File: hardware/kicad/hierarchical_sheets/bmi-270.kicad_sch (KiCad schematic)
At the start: 3 parts

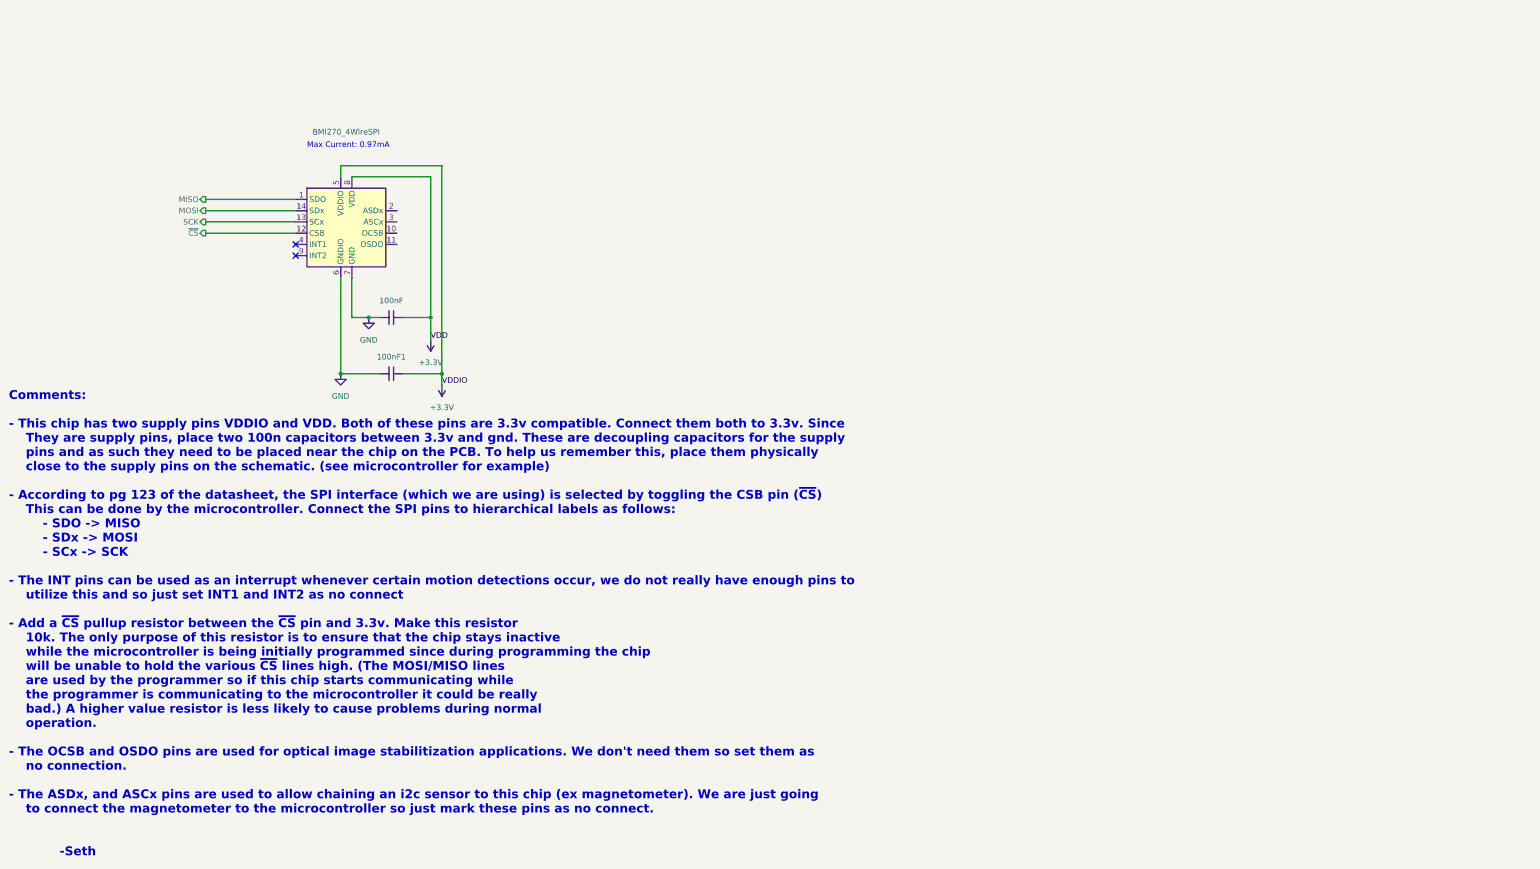
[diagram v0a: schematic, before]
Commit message: Finnished Schematic?
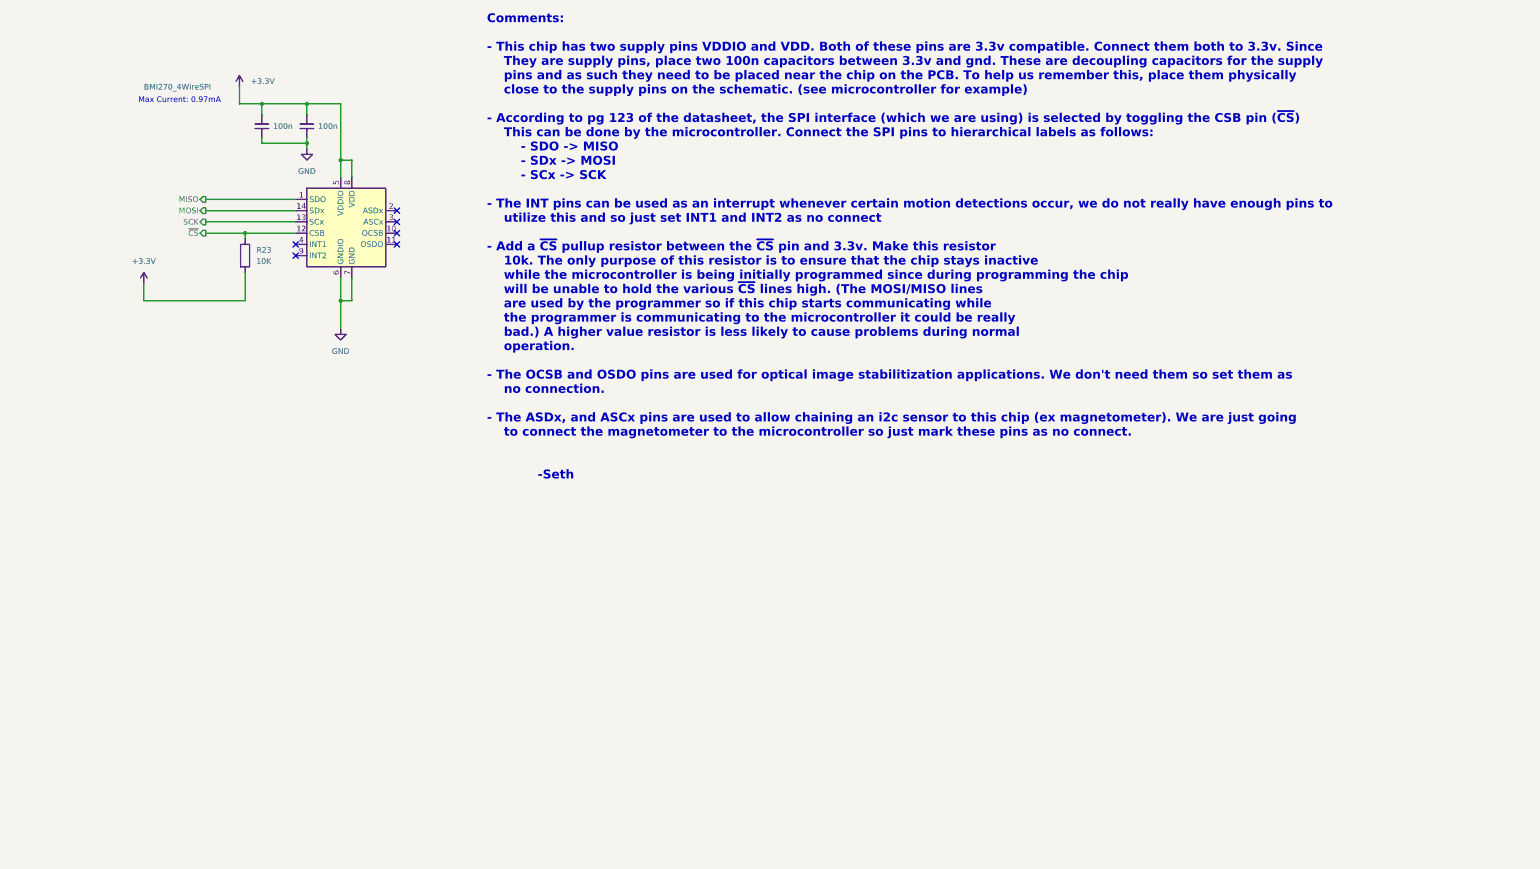
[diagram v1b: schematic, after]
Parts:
- added R23: 10K, symbol Device:R
- renumbered 100nF to 100n, 100nF1 to 100n
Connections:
- net +3.3V: now also 100n.2, 100n.2, R23.2; no longer 100n.1, 100n.1
- net GND: now also 100n.1, 100n.1; no longer 100n.2, 100n.2
- net ~{CS}: now also R23.1
- no-connect marks 2 -> 6
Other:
- moved on the sheet: 100n
